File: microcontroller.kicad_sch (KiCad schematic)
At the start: 10 parts, among them U1 ATSAMD21G18A, Y2 Crystal_GND3

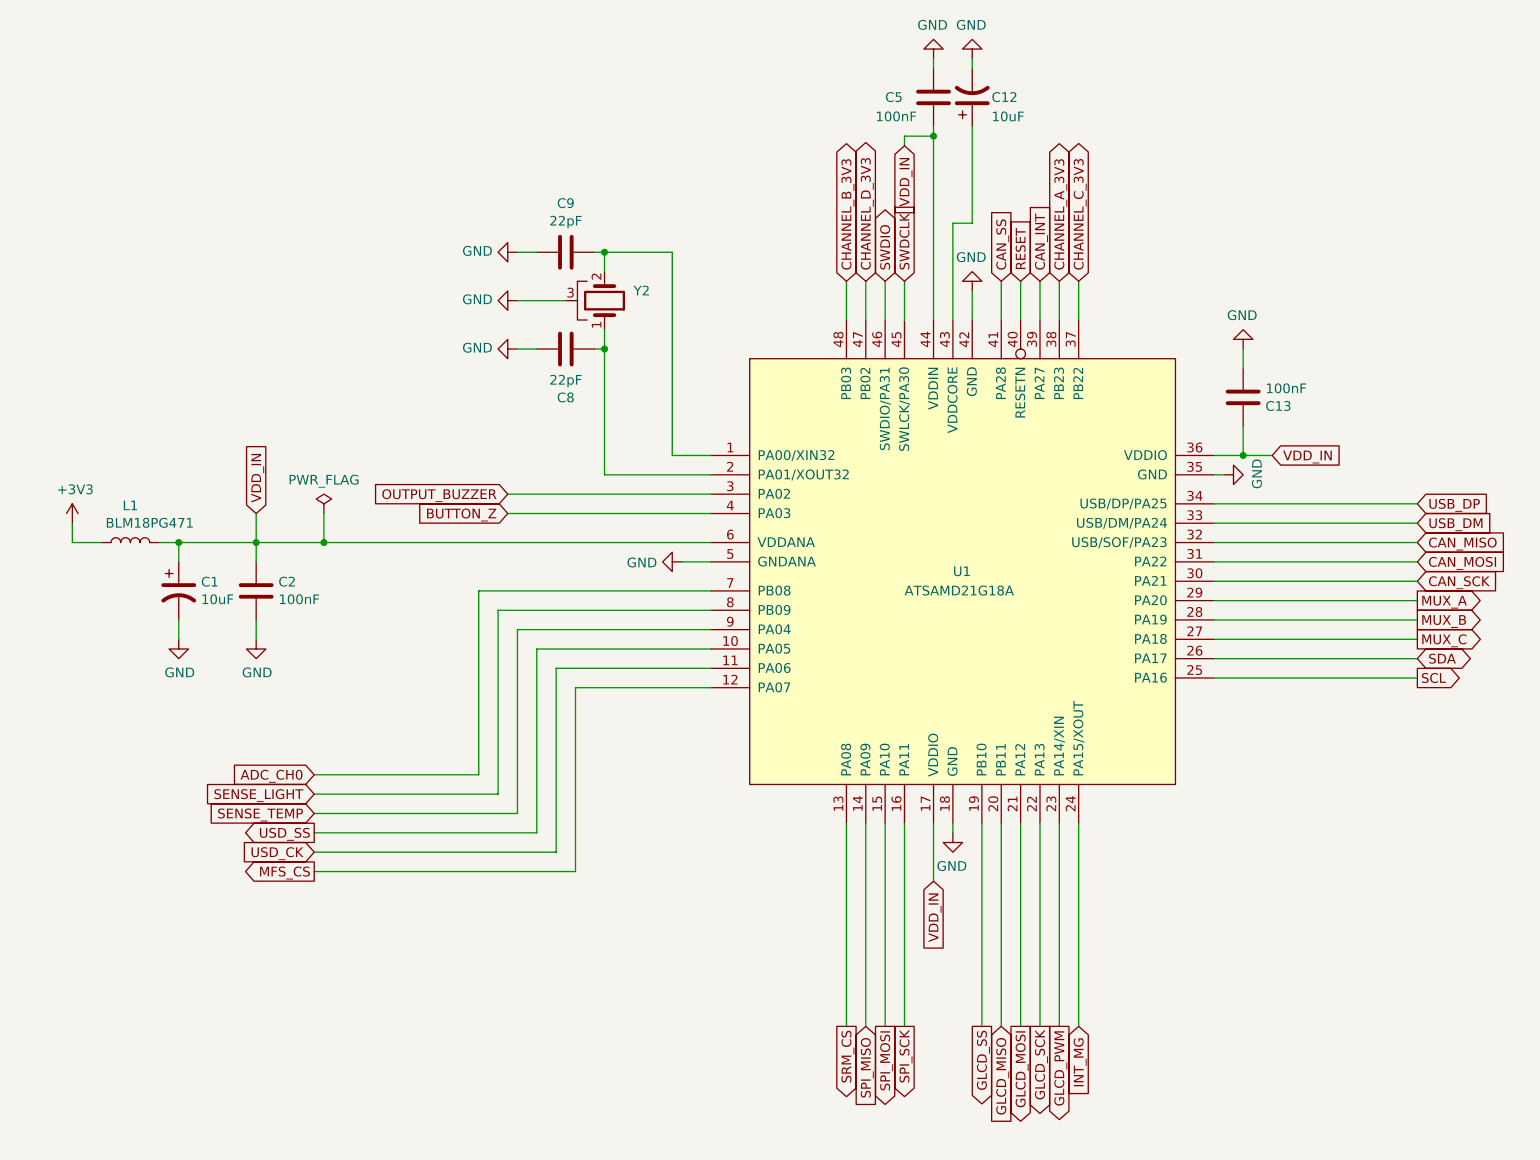
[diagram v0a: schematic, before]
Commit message: 25/01/24/A
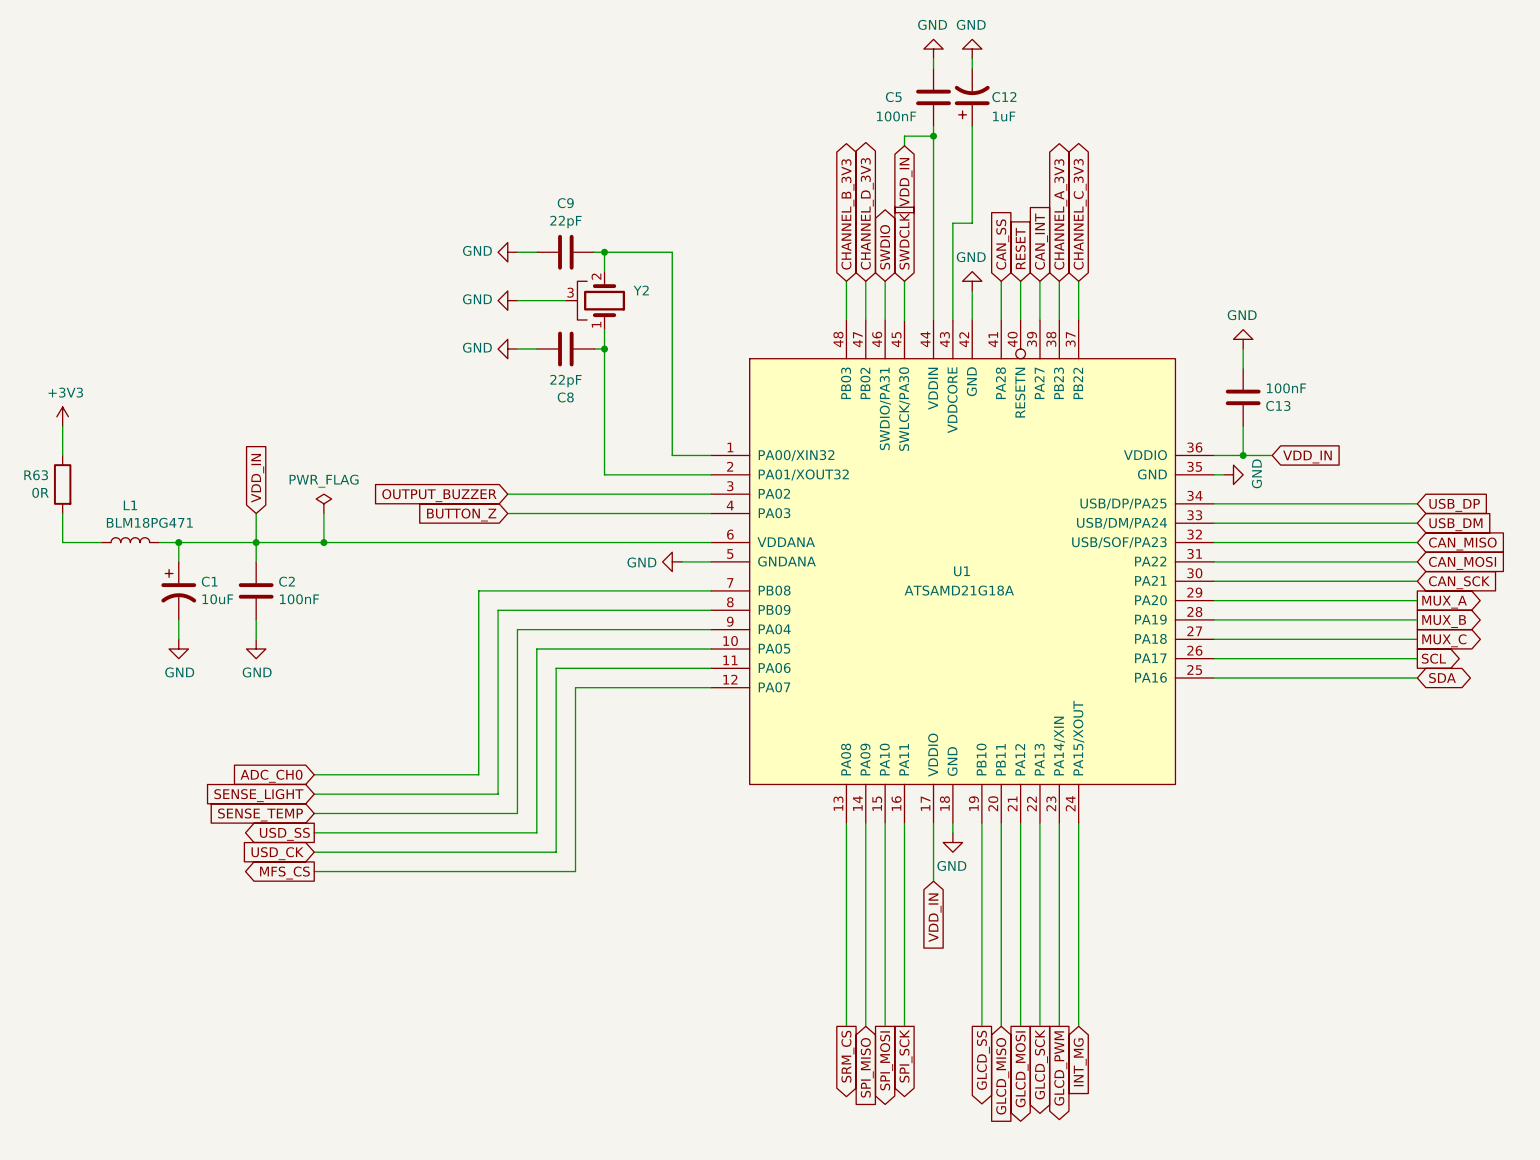
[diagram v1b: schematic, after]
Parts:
- added R63: 0R, Resistor_SMD:R_1206_3216Metric, symbol Device:R
- C12: value 10uF -> 1uF
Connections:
- net +3V3: now also R63.1; no longer L1.1
- net SCL: now also U1.26 (PA17); no longer U1.25 (PA16)
- net SDA: now also U1.25 (PA16); no longer U1.26 (PA17)
- new net: L1.1, R63.2
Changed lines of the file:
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@@
 	(wire
 		(pts
+			(xy 30.48 86.36) (xy 30.48 90.17)
+		)
+		(stroke
+			(width 0)
+			(type default)
+		)
+	)
+	(wire
+		(pts
 			(xy 181.61 85.09) (xy 208.28 85.09)
 		)
@@
 	(wire
 		(pts
+			(xy 30.48 74.93) (xy 30.48 78.74)
+		)
+		(stroke
+			(width 0)
+			(type default)
+		)
+	)
+	(wire
+		(pts
 			(xy 149.86 60.96) (xy 149.86 57.15)
 		)
@@
 	(wire
 		(pts
-			(xy 31.75 90.17) (xy 35.56 90.17)
+			(xy 30.48 90.17) (xy 35.56 90.17)
 		)
 		(stroke
@@
 	(wire
 		(pts
-			(xy 31.75 87.63) (xy 31.75 90.17)
-		)
-		(stroke
-			(width 0)
-			(type default)
-		)
-	)
-	(wire
-		(pts
 			(xy 101.6 81.28) (xy 115.57 81.28)
 		)
@@
 	(global_label "SDA"
 		(shape bidirectional)
-		(at 208.28 105.41 0)
+		(at 208.28 107.95 0)
 		(fields_autoplaced yes)
 		(effects
@@
 		)
 		(property "Intersheetrefs" "${INTERSHEET_REFS}"
-			(at 0 0 0)
+			(at 0 2.54 0)
 			(effects
 				(font
@@
 	(global_label "SCL"
 		(shape output)
-		(at 208.28 107.95 0)
+		(at 208.28 105.41 0)
 		(fields_autoplaced yes)
 		(effects
@@
 		)
 		(property "Intersheetrefs" "${INTERSHEET_REFS}"
-			(at 0 0 0)
+			(at 0 -2.54 0)
 			(effects
 				(font
@@
 	(symbol
 		(lib_id "power:+3.3V")
-		(at 31.75 87.63 0)
+		(at 30.48 74.93 0)
 		(unit 1)
 		(exclude_from_sim no)
@@
 		(dnp no)
 		(property "Reference" "#PWR01"
-			(at 31.75 91.44 0)
+			(at 30.48 78.74 0)
 			(effects
 				(font
@@
 		)
 		(property "Value" "+3V3"
-			(at 32.131 83.2358 0)
+			(at 30.861 70.5358 0)
 			(effects
 				(font
@@
 		)
 		(property "Footprint" ""
-			(at 31.75 87.63 0)
+			(at 30.48 74.93 0)
 			(effects
 				(font
@@
 		)
 		(property "Datasheet" ""
-			(at 31.75 87.63 0)
+			(at 30.48 74.93 0)
 			(effects
 				(font
@@
 		)
 		(property "Description" ""
-			(at 31.75 87.63 0)
+			(at 30.48 74.93 0)
 			(effects
 				(font
@@
 			)
 		)
-		(property "Value" "10uF"
+		(property "Value" "1uF"
 			(at 152.4 34.29 0)
 			(effects
@@
 			)
 		)
-		(property "Datasheet" ""
+		(property "Datasheet" "https://ww1.microchip.com/downloads/en/DeviceDoc/SAM-D21-DA1-Family-Data-Sheet-DS40001882H.pdf"
 			(at 156.21 101.6 0)
 			(effects
@@
 		)
 		(instances
-			(project "Game_Cat_R4"
+			(project ""
+				(path "/96315415-cfed-47d2-b3dd-d782358bd0df/00000000-0000-0000-0000-00005cbab8ae"
+					(reference "U1")
+					(unit 1)
+				)
 				(path "/96315415-cfed-47d2-b3dd-d782358bd0df/00000000-0000-0000-0000-00005ce5bb47"
 					(reference "U1")
@@
 					(unit 1)
 				)
+			)
+		)
+	)
+	(symbol
+		(lib_id "Device:R")
+		(at 30.48 82.55 0)
+		(mirror y)
+		(unit 1)
+		(exclude_from_sim no)
+		(in_bom yes)
+		(on_board yes)
+		(dnp no)
+		(property "Reference" "R63"
+			(at 28.702 81.3816 0)
+			(effects
+				(font
+					(size 1.27 1.27)
+				)
+				(justify left)
+			)
+		)
+		(property "Value" "0R"
+			(at 28.702 83.693 0)
+			(effects
+				(font
+					(size 1.27 1.27)
+				)
+				(justify left)
+			)
+		)
+		(property "Footprint" "Resistor_SMD:R_1206_3216Metric"
+			(at 32.258 82.55 90)
+			(effects
+				(font
+					(size 1.27 1.27)
+				)
+				(hide yes)
+			)
+		)
+		(property "Datasheet" "~"
+			(at 30.48 82.55 0)
+			(effects
+				(font
+					(size 1.27 1.27)
+				)
+				(hide yes)
+			)
+		)
+		(property "Description" ""
+			(at 30.48 82.55 0)
+			(effects
+				(font
+					(size 1.27 1.27)
+				)
+				(hide yes)
+			)
+		)
+		(pin "1"
+		)
+		(pin "2"
+		)
+		(instances
+			(project "Game_Cat_R4"
+				(path "/96315415-cfed-47d2-b3dd-d782358bd0df/00000000-0000-0000-0000-00005ce5bb47"
+					(reference "R63")
+					(unit 1)
+				)

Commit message: 05/25/25/A
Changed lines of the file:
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@@
 (kicad_sch
-	(version 20231120)
+	(version 20250114)
 	(generator "eeschema")
-	(generator_version "8.0")
+	(generator_version "9.0")
 	(paper "USLetter")
 	(title_block
